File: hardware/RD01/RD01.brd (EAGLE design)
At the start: 50 x 50 mm, 20 parts, among them J1 CON_TERMINAL_BLOCK_02-5MM, J2 CON_TERMINAL_BLOCK_02-5MM, J3 CON_TERMINAL_BLOCK_02-5MM, J4 CON_TERMINAL_BLOCK_02-5MM, K1 JS-M1-12V-5, K2 JS-M1-12V-5, Q1 BC337, Q2 BC337

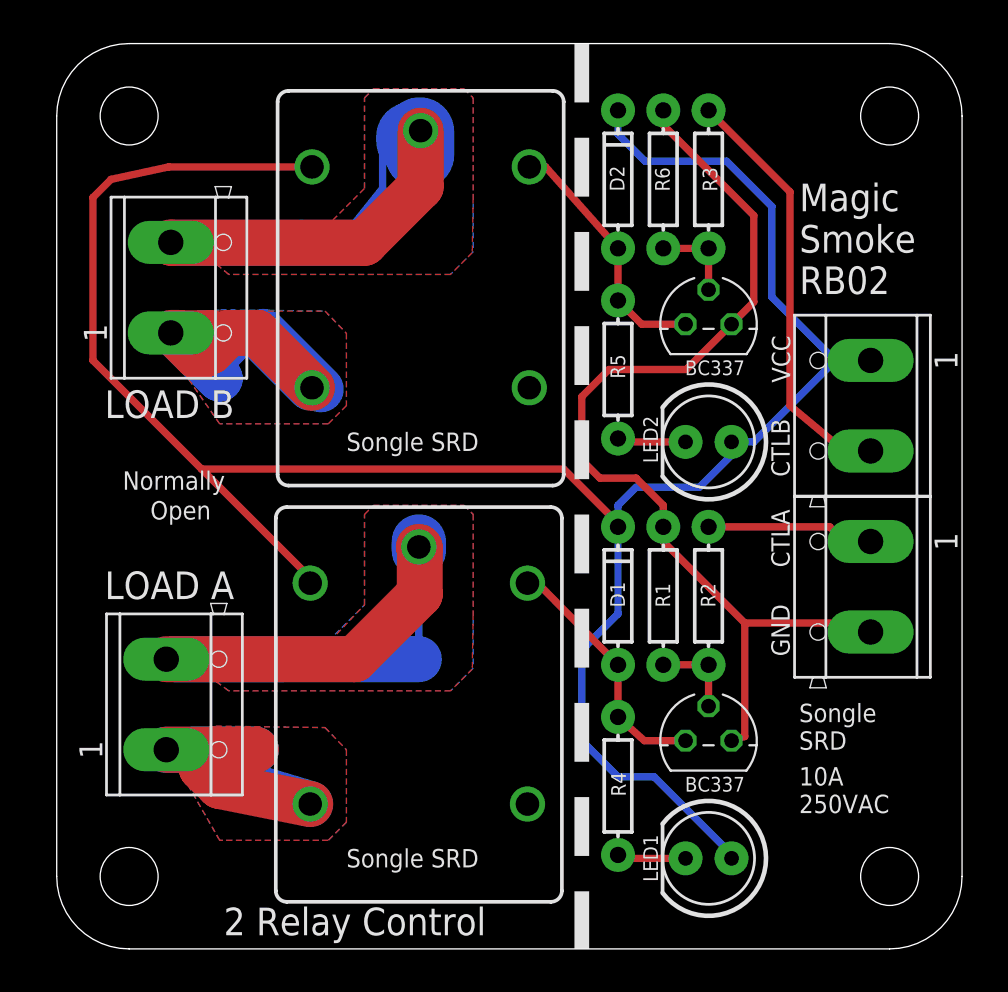
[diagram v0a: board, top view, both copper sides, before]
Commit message: RD01 Elecrow order
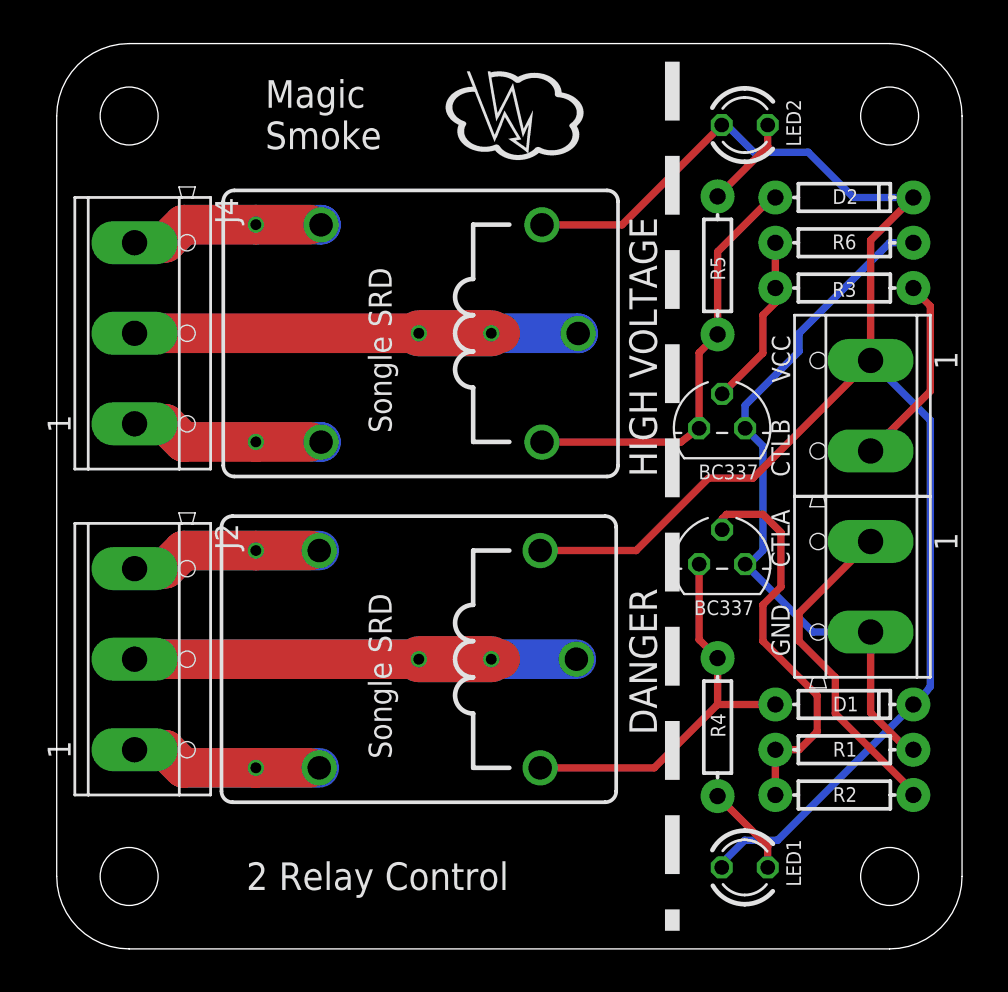
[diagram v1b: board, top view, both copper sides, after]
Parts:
- J2, J4: value CON_TERMINAL_BLOCK_02-5MM -> CON_TERMINAL_BLOCK_03-5MM; device dp_devices:TERMINAL_BLOCK_2P_5 -> dp_devices:TERMINAL_BLOCK_3P_5
- LED1, LED2: device SparkFun:LED5MM -> dp_devices:LED-3MM
- moved LED2 17.6 mm to (38.0, 45.5), turned to 0 degrees
- moved D1 13.9 mm to (43.5, 13.5), turned to 0 degrees
- moved R2 13.3 mm to (43.5, 8.50), turned to 0 degrees
- moved R1 13.1 mm to (43.5, 11.0), turned to 0 degrees
- moved D2 12.5 mm to (43.5, 41.5), turned to 0 degrees
- moved R6 10.6 mm to (43.5, 39.0), turned to 0 degrees
- moved Q1 9.78 mm to (36.8, 21.2)
- moved R3 9.60 mm to (43.5, 36.5), turned to 0 degrees
- moved R5 7.96 mm to (36.5, 37.8), turned to 90 degrees
- moved R4 6.39 mm to (36.5, 12.2)
- moved Q2 5.80 mm to (36.8, 28.8)
- moved J4 3.22 mm to (4.75, 34.0)
- moved J2 3.05 mm to (4.75, 16.0)
- moved K1 2.50 mm to (20.0, 16.0), turned to 0 degrees
- moved K2 2.50 mm to (20.1, 34.0), turned to 0 degrees
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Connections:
- net LOAD_A2 renamed LOAD_A_C
- net LOAD_B2 renamed LOAD_B_C
- removed net LOAD_A1: J2.1, K1.NO
- removed net LOAD_B1: J4.1, K2.NO
- new net LOAD_A_NC: J2.1, K1.NC
- new net LOAD_A_NO: J2.3, K1.NO
- new net LOAD_B_NC: J4.1, K2.NC
- new net LOAD_B_NO: J4.3, K2.NO
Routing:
- net LOAD_B1: track 39.4 -> 0.00 mm
- net VCC: track 127.4 -> 92.3 mm
- net LOAD_A1: track 28.7 -> 0.00 mm
- net LOAD_B_NO: track 0.00 -> 21.1 mm, vias 0 -> 1
- net LOAD_A_NC: track 0.00 -> 21.0 mm, vias 0 -> 1
- net LOAD_B_NC: track 0.00 -> 20.1 mm, vias 0 -> 1
- net LOAD_A_NO: track 0.00 -> 20.0 mm, vias 0 -> 1
- net N$6: track 4.79 -> 22.2 mm
- net GND: track 55.9 -> 39.5 mm
- net RELAY_B: track 23.5 -> 10.8 mm
- net COIL_B: track 14.1 -> 23.5 mm
- net RELAY_A: track 9.29 -> 18.2 mm
- net COIL_A: track 14.0 -> 22.6 mm
- net N$1: track 4.78 -> 9.56 mm
- net LOAD_B_C: track 41.6 -> 43.5 mm, vias 0 -> 2
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- removed copper zone on layer 1, net LOAD_A1
- removed copper zone on layer 16, net LOAD_A1
- removed copper zone on layer 1, net LOAD_A_C
- removed copper zone on layer 16, net LOAD_A_C
- removed copper zone on layer 1, net LOAD_B1
- removed copper zone on layer 16, net LOAD_B1
- removed copper zone on layer 1, net LOAD_B_C
- removed copper zone on layer 16, net LOAD_B_C
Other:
- board text added: "C"
- board text added: "Magic Smoke"
- board text added: "NC"
- board text added: "NO"
- board text added: "RD01"
- board text removed: "10A 250VAC"
- board text removed: "LOAD A"
- board text removed: "LOAD B"
- board text removed: "Magic Smoke RB02"
- board text removed: "Magic Smoke RD01"
- board text removed: "Normally"
- board text removed: "Open"
